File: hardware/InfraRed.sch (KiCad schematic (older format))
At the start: 6 parts, among them P3 CONN_01X03, U6 OPA344

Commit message: update
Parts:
- P3: footprint Pin_Headers:Pin_Header_Straight_1x03_Pitch2.54mm -> footprints:PIR-SR501
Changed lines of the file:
@@
 LIBS:contrib
 LIBS:valves
-LIBS:5v-solar-regulator-cache
-EELAYER 26 0
+LIBS:open-automation
+LIBS:5v-smart-solar-regulator-cache
+EELAYER 25 0
 EELAYER END
 $Descr A4 11693 8268
@@
 F 0 "P3" H 4350 5200 50  0000 L CNN
 F 1 "CONN_01X03" H 4350 4800 50  0001 L CNN
-F 2 "Pin_Headers:Pin_Header_Straight_1x03_Pitch2.54mm" H 4477 4904 50  0001 L CNN
+F 2 "footprints:PIR-SR501" H 4477 4904 50  0001 L CNN
 F 3 "http://sullinscorp.com/catalogs/101_PAGE114-115_.100_FEMALE_HDR.pdf" H 4400 5000 50  0001 C CNN
 	1    4400 5000
@@
 $EndComp
 $Comp
-L GND #PWR6
+L GND #PWR05
 U 1 1 59098B15
 P 4150 4850
-F 0 "#PWR6" H 4150 4600 50  0001 C CNN
+F 0 "#PWR05" H 4150 4600 50  0001 C CNN
 F 1 "GND" H 4150 4700 50  0000 C CNN
 F 2 "" H 4150 4850 50  0000 C CNN
@@
 PIR
 $Comp
-L GND #PWR7
+L GND #PWR06
 U 1 1 590BA36E
 P 4450 3150
-F 0 "#PWR7" H 4450 2900 50  0001 C CNN
+F 0 "#PWR06" H 4450 2900 50  0001 C CNN
 F 1 "GND" H 4450 3000 50  0000 C CNN
 F 2 "" H 4450 3150 50  0000 C CNN
@@
 $EndComp
 $Comp
-L GND #PWR5
+L GND #PWR07
 U 1 1 590BAE9F
 P 3750 2900
-F 0 "#PWR5" H 3750 2650 50  0001 C CNN
+F 0 "#PWR07" H 3750 2650 50  0001 C CNN
 F 1 "GND" H 3750 2750 50  0000 C CNN
 F 2 "" H 3750 2900 50  0000 C CNN

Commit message: update
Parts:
- removed U6: OPA344, TO_SOT_Packages_SMD:SOT-23-5, symbol OPA344
- added U5: OPA344NA/3K, TO_SOT_Packages_SMD:SOT-23-5, symbol OPA344NA/3K
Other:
- moved on the sheet: D3, P3, R17, R18, R19
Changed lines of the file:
@@
 LIBS:open-automation
 LIBS:5v-smart-solar-regulator-cache
-EELAYER 26 0
+EELAYER 25 0
 EELAYER END
 $Descr A4 11693 8268
@@
 L CONN_01X03 P3
 U 1 1 59098B14
-P 4400 5000
+P 7350 3900
 AR Path="/590982C4/59098B14" Ref="P3"  Part="1"
 AR Path="/59096487/59098B14" Ref="P3"  Part="1"
 AR Path="/5936D7EA/59098B14" Ref="P3"  Part="1"
-F 0 "P3" H 4350 5200 50  0000 L CNN
-F 1 "CONN_01X03" H 4350 4800 50  0001 L CNN
-F 2 "footprints:PIR-SR501" H 4477 4904 50  0001 L CNN
-F 3 "http://sullinscorp.com/catalogs/101_PAGE114-115_.100_FEMALE_HDR.pdf" H 4400 5000 50  0001 C CNN
-	1    4400 5000
+F 0 "P3" H 7300 4100 50  0000 L CNN
+F 1 "CONN_01X03" H 7300 3700 50  0001 L CNN
+F 2 "footprints:PIR-SR501" H 7427 3804 50  0001 L CNN
+F 3 "http://sullinscorp.com/catalogs/101_PAGE114-115_.100_FEMALE_HDR.pdf" H 7350 3900 50  0001 C CNN
+	1    7350 3900
 	1    0    0    -1
 $EndComp
@@
 L GND #PWR05
 U 1 1 59098B15
-P 4150 4850
-F 0 "#PWR05" H 4150 4600 50  0001 C CNN
-F 1 "GND" H 4150 4700 50  0000 C CNN
-F 2 "" H 4150 4850 50  0000 C CNN
-F 3 "" H 4150 4850 50  0000 C CNN
-	1    4150 4850
+P 7100 3750
+F 0 "#PWR05" H 7100 3500 50  0001 C CNN
+F 1 "GND" H 7100 3600 50  0000 C CNN
+F 2 "" H 7100 3750 50  0000 C CNN
+F 3 "" H 7100 3750 50  0000 C CNN
+	1    7100 3750
 	-1   0    0    1
 $EndComp
-Text GLabel 4100 5000 0    60   Input ~ 0
+Text GLabel 7050 3900 0    60   Input ~ 0
 IO16
-$Comp
-L OPA344 U6
-U 1 1 590B832C
-P 4550 2800
-F 0 "U6" H 4550 2950 50  0000 L CNN
-F 1 "OPA344" H 4500 2600 50  0000 L CNN
-F 2 "TO_SOT_Packages_SMD:SOT-23-5" H 4450 2850 50  0001 C CNN
-F 3 "http://www.digikey.com/product-detail/en/texas-instruments/OPA344NA-3K/296-41475-1-ND/5222851" H 4550 2950 50  0001 C CNN
-F 4 "296-41475-1-ND" H 4550 2800 60  0001 C CNN "Part Number"
-	1    4550 2800
-	1    0    0    -1
-$EndComp
 $Comp
 L LED D3
 U 1 1 590B85F8
-P 4000 2700
-F 0 "D3" H 4000 2800 50  0000 C CNN
-F 1 "LED" H 4000 2600 50  0000 C CNN
-F 2 "LEDs:LED_D3.0mm" H 4000 2700 50  0001 C CNN
-F 3 "http://www.ttelectronics.com/sites/default/files/download-files/OP993-999_0.pdf" H 4000 2700 50  0001 C CNN
-F 4 "365-1086-ND" H 4000 2700 60  0001 C CNN "Part Number"
-	1    4000 2700
+P 4250 3750
+F 0 "D3" H 4250 3850 50  0000 C CNN
+F 1 "LED" H 4250 3650 50  0000 C CNN
+F 2 "LEDs:LED_D3.0mm" H 4250 3750 50  0001 C CNN
+F 3 "http://www.ttelectronics.com/sites/default/files/download-files/OP993-999_0.pdf" H 4250 3750 50  0001 C CNN
+F 4 "365-1086-ND" H 4250 3750 60  0001 C CNN "Part Number"
+	1    4250 3750
 	-1   0    0    1
 $EndComp
@@
 L R R19
 U 1 1 590B885D
-P 4450 3550
-F 0 "R19" V 4530 3550 50  0000 C CNN
-F 1 "180K" V 4450 3550 50  0000 C CNN
-F 2 "Resistors_SMD:R_0603_HandSoldering" V 4380 3550 50  0001 C CNN
-F 3 "http://www.yageo.com/documents/recent/PYu-RC_Group_51_RoHS_L_7.pdf" H 4450 3550 50  0001 C CNN
-F 4 "RC0603JR-07180KL" V 4450 3550 60  0001 C CNN "Part Number"
-	1    4450 3550
+P 4700 4600
+F 0 "R19" V 4780 4600 50  0000 C CNN
+F 1 "180K" V 4700 4600 50  0000 C CNN
+F 2 "Resistors_SMD:R_0603_HandSoldering" V 4630 4600 50  0001 C CNN
+F 3 "http://www.yageo.com/documents/recent/PYu-RC_Group_51_RoHS_L_7.pdf" H 4700 4600 50  0001 C CNN
+F 4 "RC0603JR-07180KL" V 4700 4600 60  0001 C CNN "Part Number"
+	1    4700 4600
 	0    -1   -1   0
 $EndComp
@@
 L R R17
 U 1 1 590B8957
-P 4000 2900
-F 0 "R17" V 4080 2900 50  0000 C CNN
-F 1 "22K" V 4000 2900 50  0000 C CNN
-F 2 "Resistors_SMD:R_0603_HandSoldering" V 3930 2900 50  0001 C CNN
-F 3 "http://www.yageo.com/documents/recent/PYu-RC_Group_51_RoHS_L_7.pdf" H 4000 2900 50  0001 C CNN
-F 4 "RC0603JR-0722KL" V 4000 2900 60  0001 C CNN "Part Number"
-	1    4000 2900
+P 4250 3950
+F 0 "R17" V 4330 3950 50  0000 C CNN
+F 1 "22K" V 4250 3950 50  0000 C CNN
+F 2 "Resistors_SMD:R_0603_HandSoldering" V 4180 3950 50  0001 C CNN
+F 3 "http://www.yageo.com/documents/recent/PYu-RC_Group_51_RoHS_L_7.pdf" H 4250 3950 50  0001 C CNN
+F 4 "RC0603JR-0722KL" V 4250 3950 60  0001 C CNN "Part Number"
+	1    4250 3950
 	0    1    1    0
 $EndComp
@@
 L R R18
 U 1 1 590B8E6E
-P 4200 2400
-F 0 "R18" V 4280 2400 50  0000 C CNN
-F 1 "1M" V 4200 2400 50  0000 C CNN
-F 2 "Resistors_SMD:R_0603_HandSoldering" V 4130 2400 50  0001 C CNN
-F 3 "http://www.yageo.com/documents/recent/PYu-RC_Group_51_RoHS_L_7.pdf" H 4200 2400 50  0001 C CNN
-F 4 "RC0603FR-071ML" V 4200 2400 60  0001 C CNN "Part Number"
-	1    4200 2400
+P 4450 3450
+F 0 "R18" V 4530 3450 50  0000 C CNN
+F 1 "1M" V 4450 3450 50  0000 C CNN
+F 2 "Resistors_SMD:R_0603_HandSoldering" V 4380 3450 50  0001 C CNN
+F 3 "http://www.yageo.com/documents/recent/PYu-RC_Group_51_RoHS_L_7.pdf" H 4450 3450 50  0001 C CNN
+F 4 "RC0603FR-071ML" V 4450 3450 60  0001 C CNN "Part Number"
+	1    4450 3450
 	-1   0    0    1
 $EndComp
-Text GLabel 5050 2800 2    60   Input ~ 0
+Text GLabel 5300 3850 2    60   Input ~ 0
 IO34
-Text Label 4250 1750 0    60   ~ 0
+Text Label 4500 2800 0    60   ~ 0
 Light-Level
-Text Label 4050 4550 0    60   ~ 0
+Text Label 7000 3450 0    60   ~ 0
 PIR
 $Comp
 L GND #PWR06
 U 1 1 590BA36E
-P 4450 3150
-F 0 "#PWR06" H 4450 2900 50  0001 C CNN
-F 1 "GND" H 4450 3000 50  0000 C CNN
-F 2 "" H 4450 3150 50  0000 C CNN
-F 3 "" H 4450 3150 50  0000 C CNN
-	1    4450 3150
+P 4700 4200
+F 0 "#PWR06" H 4700 3950 50  0001 C CNN
+F 1 "GND" H 4700 4050 50  0000 C CNN
+F 2 "" H 4700 4200 50  0000 C CNN
+F 3 "" H 4700 4200 50  0000 C CNN
+	1    4700 4200
 	1    0    0    -1
 $EndComp
@@
 L GND #PWR07
 U 1 1 590BAE9F
-P 3750 2900
-F 0 "#PWR07" H 3750 2650 50  0001 C CNN
-F 1 "GND" H 3750 2750 50  0000 C CNN
-F 2 "" H 3750 2900 50  0000 C CNN
-F 3 "" H 3750 2900 50  0000 C CNN
-	1    3750 2900
+P 4000 3950
+F 0 "#PWR07" H 4000 3700 50  0001 C CNN
+F 1 "GND" H 4000 3800 50  0000 C CNN
+F 2 "" H 4000 3950 50  0000 C CNN
+F 3 "" H 4000 3950 50  0000 C CNN
+	1    4000 3950
 	0    1    1    0
 $EndComp
 Wire Wire Line
-	4150 4850 4150 4900
+	7100 3750 7100 3800
 Wire Wire Line
-	4150 4900 4200 4900
+	7100 3800 7150 3800
 Wire Wire Line
-	4200 5100 4150 5100
+	7150 4000 7100 4000
 Wire Wire Line
-	4150 5100 4150 5150
+	7100 4000 7100 4050
 Wire Wire Line
-	4100 5000 4200 5000
+	7050 3900 7150 3900
 Wire Wire Line
-	4850 2800 5050 2800
+	5100 3850 5300 3850
 Wire Wire Line
-	4450 3100 4450 3150
+	4700 4150 4700 4200
 Wire Wire Line
-	4450 2100 4450 2500
+	4700 3150 4700 3550
 Wire Wire Line
-	4150 2900 4250 2900
+	4400 3950 4500 3950
 Wire Wire Line
-	3750 2900 3850 2900
+	4000 3950 4100 3950
 Wire Wire Line
-	3850 2700 3800 2700
+	4100 3750 4050 3750
 Wire Wire Line
-	3800 2700 3800 2900
-Connection ~ 3800 2900
+	4050 3750 4050 3950
+Connection ~ 4050 3950
 Wire Wire Line
-	4600 3550 4950 3550
+	4850 4600 5200 4600
 Wire Wire Line
-	4950 3550 4950 2800
-Connection ~ 4950 2800
+	5200 4600 5200 3850
+Connection ~ 5200 3850
 Wire Wire Line
-	4300 3550 4200 3550
+	4550 4600 4450 4600
 Wire Wire Line
-	4200 3550 4200 2900
-Connection ~ 4200 2900
+	4450 4600 4450 3950
+Connection ~ 4450 3950
 Wire Wire Line
-	4150 2700 4250 2700
+	4400 3750 4500 3750
 Wire Wire Line
-	4200 2550 4200 2700
-Connection ~ 4200 2700
+	4450 3600 4450 3750
+Connection ~ 4450 3750
 Wire Wire Line
-	4200 2250 4200 2200
+	4450 3300 4450 3250
 Wire Wire Line
-	4200 2200 4450 2200
-Connection ~ 4450 2200
-Text GLabel 4450 2100 1    60   Input ~ 0
+	4450 3250 4700 3250
+Connection ~ 4700 3250
+Text GLabel 4700 3150 1    60   Input ~ 0
 5V
-Text GLabel 4150 5150 3    60   Input ~ 0
+Text GLabel 7100 4050 3    60   Input ~ 0
 5V
+$Comp
+L OPA344NA/3K U5
+U 1 1 598F7921
+P 4800 3850
+F 0 "U5" H 4800 4100 50  0000 L CNN
+F 1 "OPA344NA/3K" H 4800 4000 50  0000 L CNN
+F 2 "TO_SOT_Packages_SMD:SOT-23-5" H 4800 3700 50  0001 L CNN
+F 3 "https://www.digikey.com/product-detail/en/texas-instruments/OPA344NA-3K/296-41475-1-ND/5222851" H 4950 4000 50  0001 C CNN
+F 4 "OPA344NA/3K" H 4800 3850 60  0001 C CNN "Part Number"
+	1    4800 3850
+	1    0    0    -1
+$EndComp
 $EndSCHEMATC

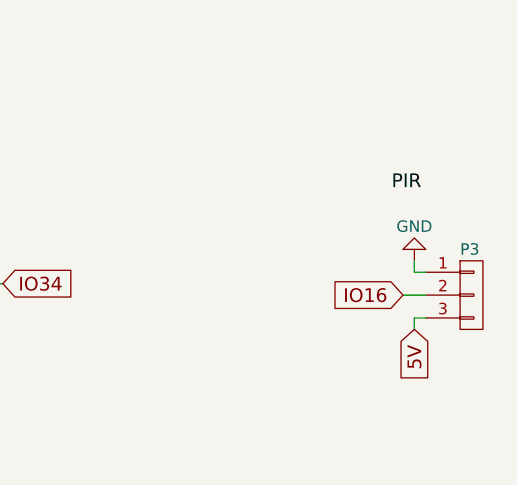
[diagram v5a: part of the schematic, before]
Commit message: update
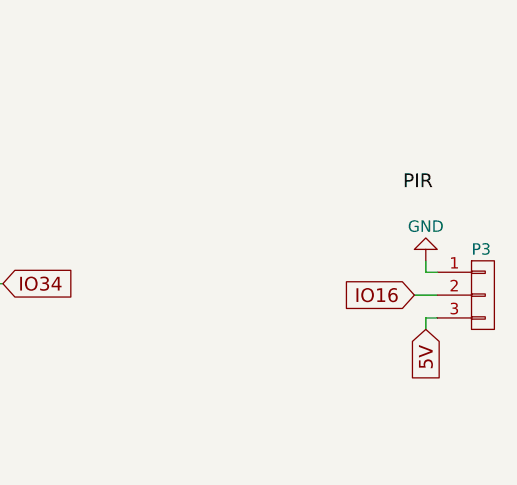
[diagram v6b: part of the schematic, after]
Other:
- moved on the sheet: P3
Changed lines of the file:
@@
 LIBS:contrib
 LIBS:valves
-LIBS:5v-smart-solar-regulator-cache
+LIBS:open-automation
+LIBS:smart-regulator-cache
 EELAYER 25 0
 EELAYER END
 $Descr A4 11693 8268
 encoding utf-8
-Sheet 3 6
+Sheet 3 7
 Title ""
 Date ""
@@
 L CONN_01X03 P3
 U 1 1 59098B14
-P 7350 3900
+P 7400 3900
 AR Path="/590982C4/59098B14" Ref="P3"  Part="1"
 AR Path="/59096487/59098B14" Ref="P3"  Part="1"
 AR Path="/5936D7EA/59098B14" Ref="P3"  Part="1"
-F 0 "P3" H 7300 4100 50  0000 L CNN
-F 1 "CONN_01X03" H 7300 3700 50  0001 L CNN
-F 2 "footprints:PIR-SR501" H 7427 3804 50  0001 L CNN
-F 3 "http://sullinscorp.com/catalogs/101_PAGE114-115_.100_FEMALE_HDR.pdf" H 7350 3900 50  0001 C CNN
-	1    7350 3900
+F 0 "P3" H 7350 4100 50  0000 L CNN
+F 1 "CONN_01X03" H 7350 3700 50  0001 L CNN
+F 2 "footprints:PIR-SR501" H 7477 3804 50  0001 L CNN
+F 3 "http://sullinscorp.com/catalogs/101_PAGE114-115_.100_FEMALE_HDR.pdf" H 7400 3900 50  0001 C CNN
+	1    7400 3900
 	1    0    0    -1
 $EndComp
@@
 L GND #PWR05
 U 1 1 59098B15
-P 7100 3750
-F 0 "#PWR05" H 7100 3500 50  0001 C CNN
-F 1 "GND" H 7100 3600 50  0000 C CNN
-F 2 "" H 7100 3750 50  0000 C CNN
-F 3 "" H 7100 3750 50  0000 C CNN
-	1    7100 3750
+P 7150 3750
+F 0 "#PWR05" H 7150 3500 50  0001 C CNN
+F 1 "GND" H 7150 3600 50  0000 C CNN
+F 2 "" H 7150 3750 50  0000 C CNN
+F 3 "" H 7150 3750 50  0000 C CNN
+	1    7150 3750
 	-1   0    0    1
 $EndComp
-Text GLabel 7050 3900 0    60   Input ~ 0
+Text GLabel 7100 3900 0    60   Input ~ 0
 IO16
 $Comp
@@
 Text Label 4500 2800 0    60   ~ 0
 Light-Level
-Text Label 7000 3450 0    60   ~ 0
+Text Label 7050 3450 0    60   ~ 0
 PIR
 $Comp
@@
 $EndComp
 Wire Wire Line
-	7100 3750 7100 3800
+	7150 3750 7150 3800
 Wire Wire Line
-	7100 3800 7150 3800
+	7150 3800 7200 3800
 Wire Wire Line
-	7150 4000 7100 4000
+	7200 4000 7150 4000
 Wire Wire Line
-	7100 4000 7100 4050
+	7150 4000 7150 4050
 Wire Wire Line
-	7050 3900 7150 3900
+	7100 3900 7200 3900
 Wire Wire Line
 	5100 3850 5300 3850
@@
 Text GLabel 4700 3150 1    60   Input ~ 0
 5V
-Text GLabel 7100 4050 3    60   Input ~ 0
+Text GLabel 7150 4050 3    60   Input ~ 0
 5V
 $Comp
